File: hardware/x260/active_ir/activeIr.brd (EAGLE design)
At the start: 11.1 x 16.5 mm, 8 parts, among them Q1 MOSFET-N

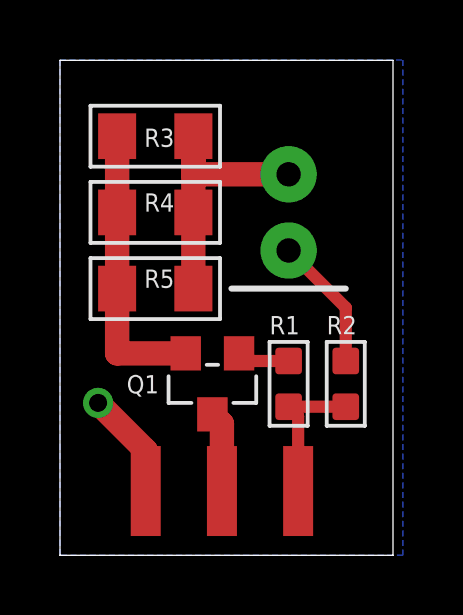
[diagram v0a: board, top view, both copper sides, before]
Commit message: Initial simulation implementation
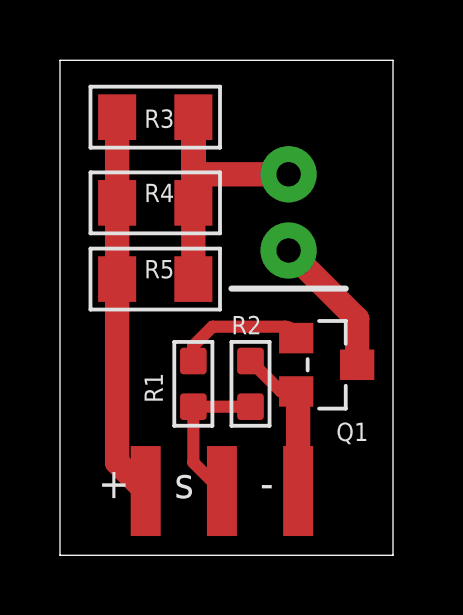
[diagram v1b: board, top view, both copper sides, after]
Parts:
- moved Q1 3.86 mm to (8.89, 6.35), turned to 270 degrees
- moved R2 3.18 mm to (6.35, 5.71)
- moved R1 3.17 mm to (4.45, 5.71)
- moved R3 0.63 mm to (3.17, 14.6)
- moved R4 0.32 mm to (3.17, 11.7)
- moved R5 0.32 mm to (3.17, 9.21)
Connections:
- net GND: now also J1.3, Q1.2; no longer D1.K, J1.1
- net N$1: now also D1.K, Q1.3; no longer Q1.2, R3.2, R4.2, R5.1
- net SIGNAL: now also J1.2; no longer J1.3
- net VCC: now also J1.1, R3.2, R4.2, R5.1; no longer J1.2, Q1.3
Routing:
- net VCC: track 2.69 -> 12.9 mm
- net N$1: track 9.53 -> 4.76 mm
- net GND: track 8.07 -> 5.29 mm, vias 1 -> 0
- net N$2: track 1.90 -> 4.36 mm
- net N$3: track 9.53 -> 10.5 mm
- removed copper zone on layer 16, net GND
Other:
- board text added: "+"
- board text added: "-"
- board text added: "s"
